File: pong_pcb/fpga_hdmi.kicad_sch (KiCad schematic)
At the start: 10 parts, among them J2 685119134923, U3 TPD12S016RKTR

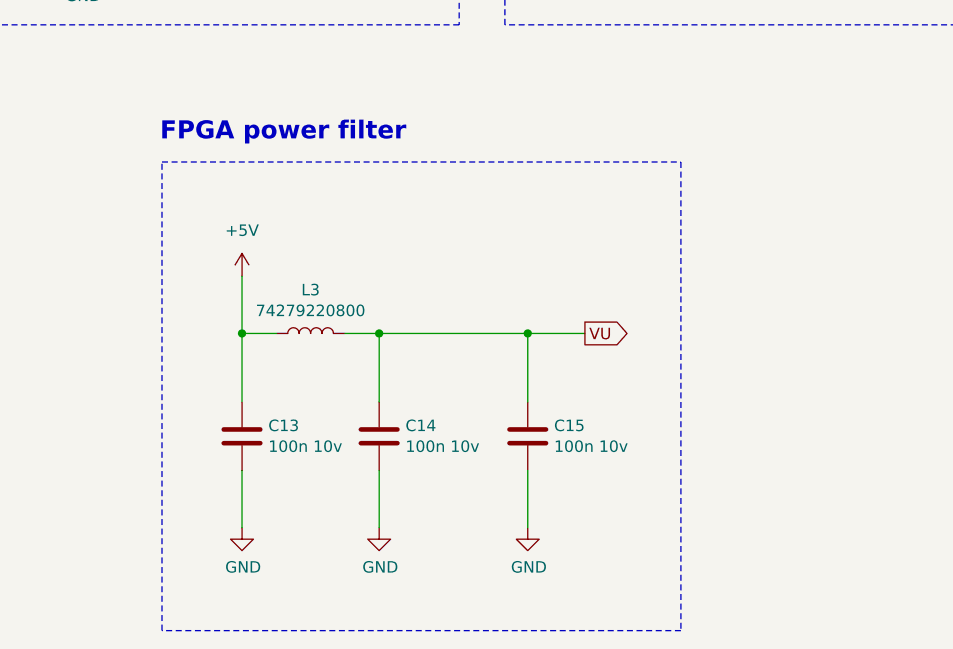
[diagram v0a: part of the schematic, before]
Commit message: Update schema and route PCB
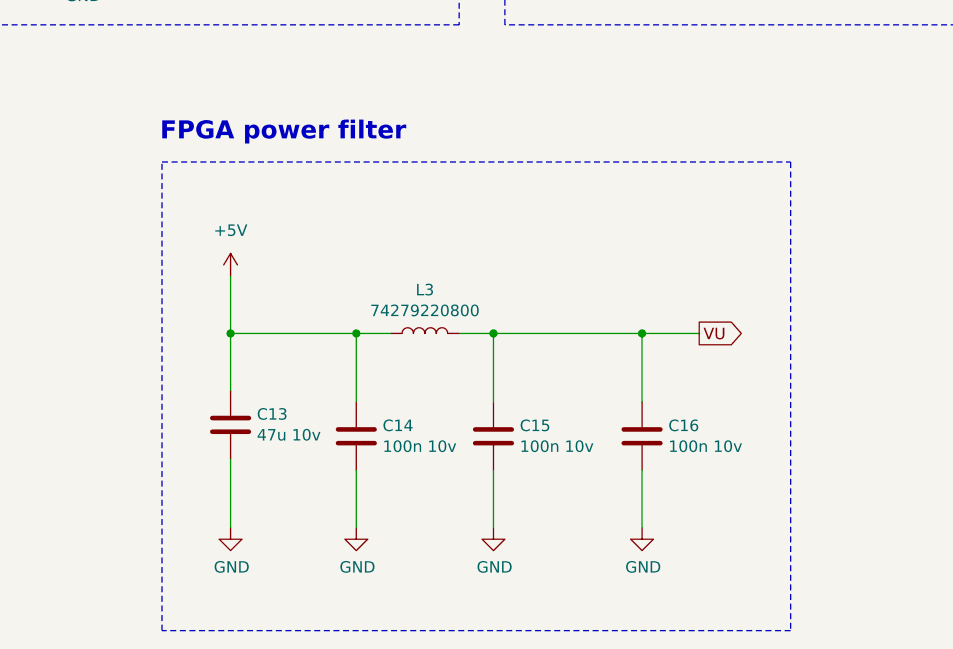
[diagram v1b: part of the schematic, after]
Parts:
- added C13: 47u 10v, Capacitor_SMD:C_1206_3216Metric_Pad1.33x1.80mm_HandSolder, symbol Device:C
- renumbered C13 to C14, C14 to C15, C15 to C16
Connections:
- net +5V: now also C13.1
- net GND: now also C13.2
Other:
- moved on the sheet: C14, C15, C16, L3

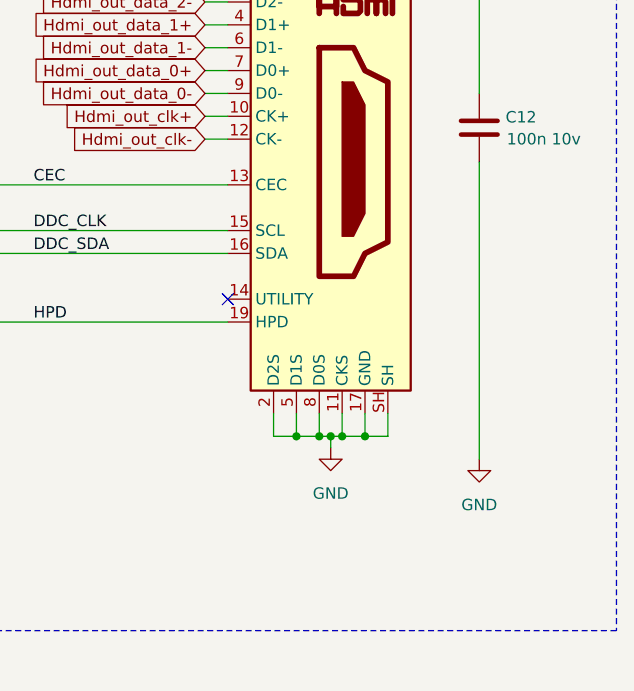
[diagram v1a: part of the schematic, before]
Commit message: Other connectors
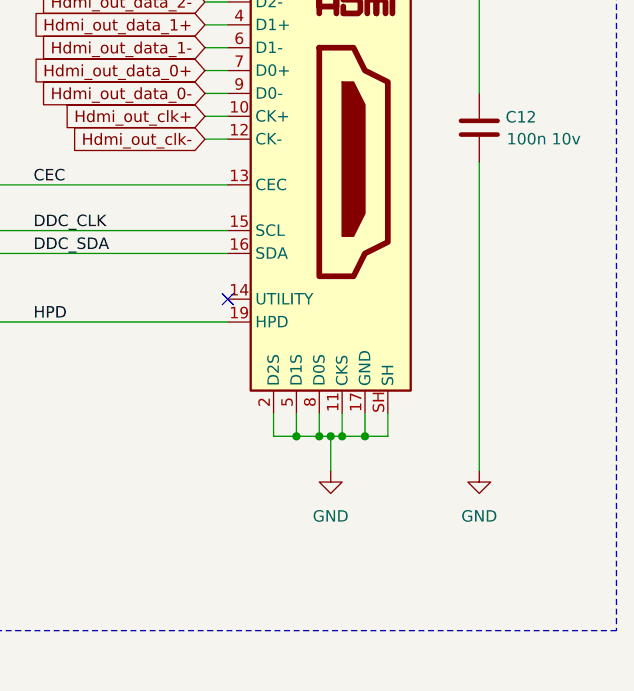
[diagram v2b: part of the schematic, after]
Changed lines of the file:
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@@
 	(wire
 		(pts
-			(xy 265.43 66.04) (xy 265.43 99.06)
+			(xy 265.43 66.04) (xy 265.43 100.33)
 		)
 		(stroke
@@
 	(wire
 		(pts
-			(xy 248.92 96.52) (xy 248.92 97.79)
+			(xy 248.92 96.52) (xy 248.92 100.33)
 		)
 		(stroke
@@
 	(symbol
 		(lib_id "power:GND")
-		(at 248.92 97.79 0)
+		(at 248.92 100.33 0)
 		(unit 1)
 		(exclude_from_sim no)
@@
 		(fields_autoplaced yes)
 		(property "Reference" "#PWR025"
-			(at 248.92 104.14 0)
+			(at 248.92 106.68 0)
 			(effects
 				(font
@@
 		)
 		(property "Value" "GND"
-			(at 248.92 102.87 0)
+			(at 248.92 105.41 0)
 			(effects
 				(font
@@
 		)
 		(property "Footprint" ""
-			(at 248.92 97.79 0)
+			(at 248.92 100.33 0)
 			(effects
 				(font
@@
 		)
 		(property "Datasheet" ""
-			(at 248.92 97.79 0)
+			(at 248.92 100.33 0)
 			(effects
 				(font
@@
 		)
 		(property "Description" "Power symbol creates a global label with name \"GND\" , ground"
-			(at 248.92 97.79 0)
+			(at 248.92 100.33 0)
 			(effects
 				(font
@@
 	(symbol
 		(lib_id "power:GND")
-		(at 265.43 99.06 0)
+		(at 265.43 100.33 0)
 		(unit 1)
 		(exclude_from_sim no)
@@
 		(fields_autoplaced yes)
 		(property "Reference" "#PWR026"
+			(at 265.43 106.68 0)
+			(effects
+				(font
+					(size 1.27 1.27)
+				)
+				(hide yes)
+			)
+		)
+		(property "Value" "GND"
 			(at 265.43 105.41 0)
 			(effects
@@
 					(size 1.27 1.27)
 				)
-				(hide yes)
-			)
-		)
-		(property "Value" "GND"
-			(at 265.43 104.14 0)
-			(effects
-				(font
-					(size 1.27 1.27)
-				)
 			)
 		)
 		(property "Footprint" ""
-			(at 265.43 99.06 0)
+			(at 265.43 100.33 0)
 			(effects
 				(font
@@
 		)
 		(property "Datasheet" ""
-			(at 265.43 99.06 0)
+			(at 265.43 100.33 0)
 			(effects
 				(font
@@
 		)
 		(property "Description" "Power symbol creates a global label with name \"GND\" , ground"
-			(at 265.43 99.06 0)
-			(effects
-				(font
+			(at 265.43 100.33 0)
+			(effects
+				(font
